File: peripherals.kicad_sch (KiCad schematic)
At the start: 32 parts, among them J5 DB25_Male_MountingHoles, J6 Conn_02x08_Odd_Even, U16 ISL83485IBZ, U27 ZXTR2012Z-7, U29 LM358

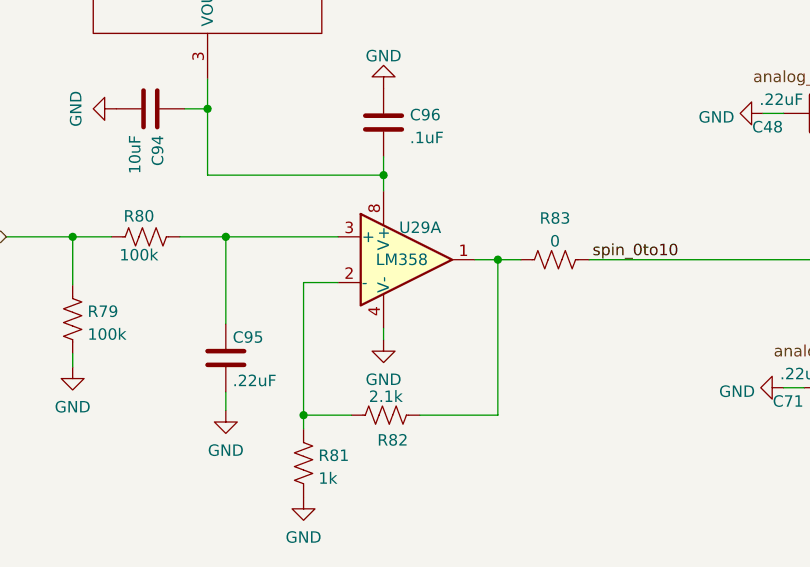
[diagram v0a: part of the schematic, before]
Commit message: removed autosave file and corrected schematic electrical rules check warnings and errors
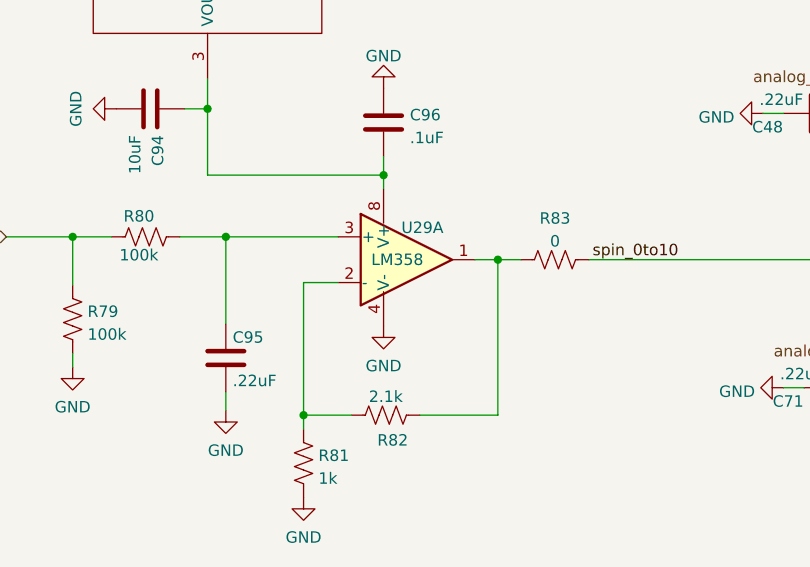
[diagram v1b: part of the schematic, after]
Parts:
- removed U29: LM358, Package_SO:SOIC-8_3.9x4.9mm_P1.27mm, symbol Amplifier_Operational:LM358
- added U29: LM358, symbol 1LibBBCTRL:LM358
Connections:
- net GND: now also U29.4 (V-)
- net at R82.2, R83.1: now also U29.1
- net at R81.2, R82.1: now also U29.2 (-)
- net at C95.1, R80.2: now also U29.3 (+)
- net at C94.1, C96.1, U27.3 (VOUT): now also U29.8 (V+)
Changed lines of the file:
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@@
   (junction (at 155.702 66.802) (diameter 0) (color 0 0 0 0)
   )
+  (junction (at 193.04 92.71) (diameter 0) (color 0 0 0 0)
+  )
   (junction (at 173.482 85.344) (diameter 0) (color 0 0 0 0)
   )
@@
   )
   (junction (at 109.982 94.996) (diameter 0) (color 0 0 0 0)
-  )
-  (junction (at 193.04 92.71) (diameter 0) (color 0 0 0 0)
   )
   (junction (at 142.24 33.274) (diameter 0) (color 0 0 0 0)
@@
     (stroke (width 0) (type default) (color 0 0 0 0))
   )
-  (wire (pts (xy 193.04 110.998) (xy 193.04 109.728))
-    (stroke (width 0) (type default) (color 0 0 0 0))
-  )
   (wire (pts (xy 75.438 36.83) (xy 82.55 36.83))
     (stroke (width 0) (type default) (color 0 0 0 0))
@@
     (stroke (width 0) (type default) (color 0 0 0 0))
   )
-  (wire (pts (xy 193.04 92.71) (xy 193.04 94.488))
-    (stroke (width 0) (type default) (color 0 0 0 0))
-  )
   (wire (pts (xy 74.168 34.29) (xy 85.852 34.29))
     (stroke (width 0) (type default) (color 0 0 0 0))
@@
   )
   (wire (pts (xy 158.496 99.568) (xy 158.496 104.902))
+    (stroke (width 0) (type default) (color 0 0 0 0))
+  )
+  (wire (pts (xy 193.04 92.71) (xy 193.04 94.234))
     (stroke (width 0) (type default) (color 0 0 0 0))
   )
@@
     (effects (font (size 1.27 1.27)) (justify right))
   )
-  (symbol (lib_id "Amplifier_Operational:LM358") (at 195.58 102.108 0) (unit 1)
-    (in_bom yes) (on_board yes)
-    (property "Reference" "U29" (id 0) (at 197.104 98.552 0))
-    (property "Value" "LM358" (id 1) (at 195.072 102.108 0))
-    (property "Footprint" "Package_SO:SOIC-8_3.9x4.9mm_P1.27mm" (id 2) (at 195.58 102.108 0)
+  (symbol (lib_id "1LibBBCTRL:LM358") (at 195.58 102.108 0) (unit 1)
+    (in_bom yes) (on_board yes)
+    (property "Reference" "U29" (id 0) (at 197.358 98.552 0))
+    (property "Value" "LM358" (id 1) (at 194.564 102.108 0))
+    (property "Footprint" "" (id 2) (at 195.58 102.108 0)
       (effects (font (size 1.27 1.27)) hide)
     )
@@
     (pin "2")
   )
+  (symbol (lib_id "1LibBBCTRL:LM358") (at 195.58 101.854 0) (unit 3)
+    (in_bom yes) (on_board yes) (fields_autoplaced)
+    (property "Reference" "U29" (id 0) (at 193.675 101.0193 0)
+      (effects (font (size 1.27 1.27)) (justify left) hide)
+    )
+    (property "Value" "LM358" (id 1) (at 193.675 103.5562 0)
+      (effects (font (size 1.27 1.27)) (justify left) hide)
+    )
+    (property "Footprint" "" (id 2) (at 195.58 101.854 0)
+      (effects (font (size 1.27 1.27)) hide)
+    )
+    (property "Datasheet" "http://www.ti.com/lit/ds/symlink/lm2904-n.pdf" (id 3) (at 195.58 101.854 0)
+      (effects (font (size 1.27 1.27)) hide)
+    )
+    (pin "1")
+    (pin "2")
+    (pin "3")
+    (pin "5")
+    (pin "6")
+    (pin "7")
+    (pin "4")
+    (pin "8")
+  )
   (symbol (lib_id "power:GND") (at 237.49 116.332 270) (unit 1)
     (in_bom yes) (on_board yes) (fields_autoplaced)
@@
     (pin "1")
   )
-  (symbol (lib_id "Amplifier_Operational:LM358") (at 195.58 102.108 0) (unit 3)
-    (in_bom yes) (on_board yes) (fields_autoplaced)
-    (property "Reference" "U29" (id 0) (at 193.675 101.2733 0)
-      (effects (font (size 1.27 1.27)) (justify left) hide)
-    )
-    (property "Value" "LM358" (id 1) (at 193.675 103.8102 0)
-      (effects (font (size 1.27 1.27)) (justify left) hide)
-    )
-    (property "Footprint" "Package_SO:SOIC-8_3.9x4.9mm_P1.27mm" (id 2) (at 195.58 102.108 0)
-      (effects (font (size 1.27 1.27)) hide)
-    )
-    (property "Datasheet" "http://www.ti.com/lit/ds/symlink/lm2904-n.pdf" (id 3) (at 195.58 102.108 0)
-      (effects (font (size 1.27 1.27)) hide)
-    )
-    (pin "1")
-    (pin "2")
-    (pin "3")
-    (pin "5")
-    (pin "6")
-    (pin "7")
-    (pin "4")
-    (pin "8")
-  )
   (symbol (lib_id "power:GND") (at 142.24 24.892 180) (unit 1)
     (in_bom yes) (on_board yes) (fields_autoplaced)
@@
     (pin "2")
   )
-  (symbol (lib_id "power:GND") (at 193.04 110.998 0) (unit 1)
-    (in_bom yes) (on_board yes) (fields_autoplaced)
-    (property "Reference" "#PWR0218" (id 0) (at 193.04 117.348 0)
-      (effects (font (size 1.27 1.27)) hide)
-    )
-    (property "Value" "GND" (id 1) (at 193.04 115.4414 0))
-    (property "Footprint" "" (id 2) (at 193.04 110.998 0)
-      (effects (font (size 1.27 1.27)) hide)
-    )
-    (property "Datasheet" "" (id 3) (at 193.04 110.998 0)
-      (effects (font (size 1.27 1.27)) hide)
-    )
+  (symbol (lib_id "power:GND") (at 193.04 109.474 0) (unit 1)
+    (in_bom yes) (on_board yes) (fields_autoplaced)
+    (property "Reference" "#PWR0218" (id 0) (at 193.04 115.824 0)
+      (effects (font (size 1.27 1.27)) hide)
+    )
+    (property "Value" "GND" (id 1) (at 193.04 113.9174 0))
+    (property "Footprint" "" (id 2) (at 193.04 109.474 0)
+      (effects (font (size 1.27 1.27)) hide)
+    )
+    (property "Datasheet" "" (id 3) (at 193.04 109.474 0)
+      (effects (font (size 1.27 1.27)) hide)
+    )
